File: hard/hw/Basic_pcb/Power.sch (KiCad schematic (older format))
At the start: 57 parts, among them P3 CONN_02X02, P4 CONN_02X02, U2 TPS63070

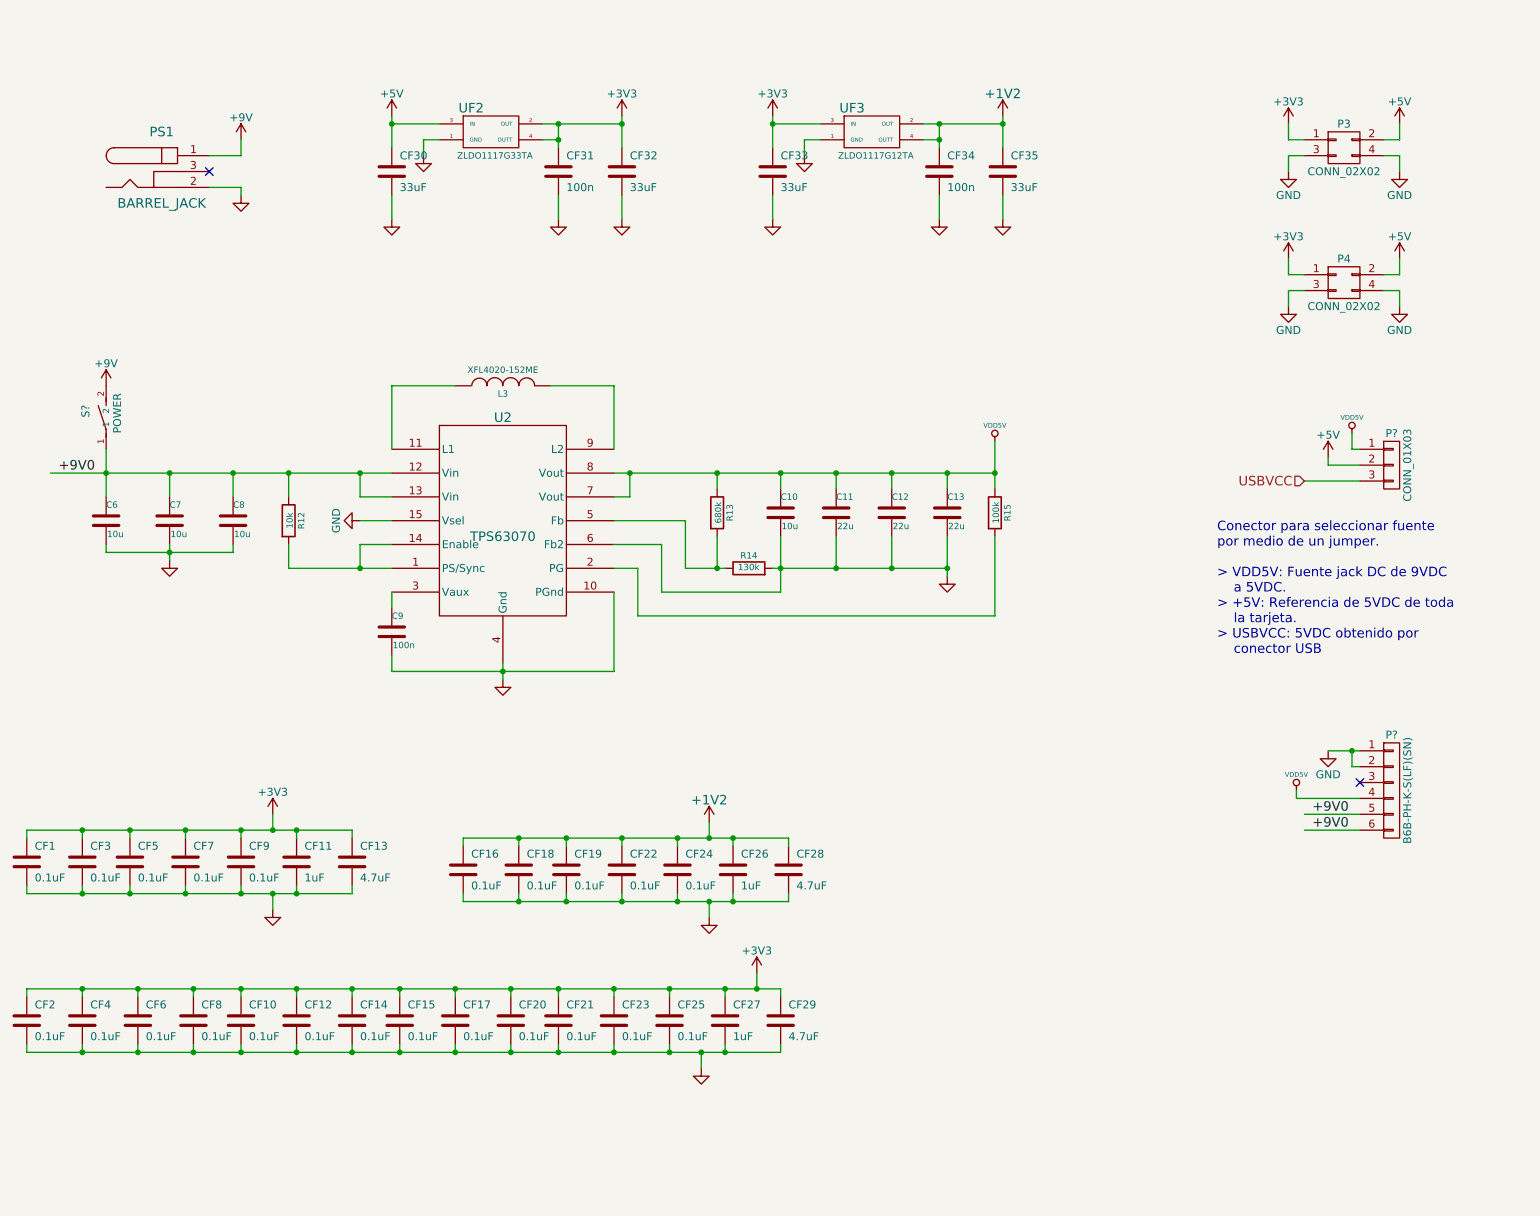
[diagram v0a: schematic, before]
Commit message: Todos los componentes en la tarjeta
by Ruben
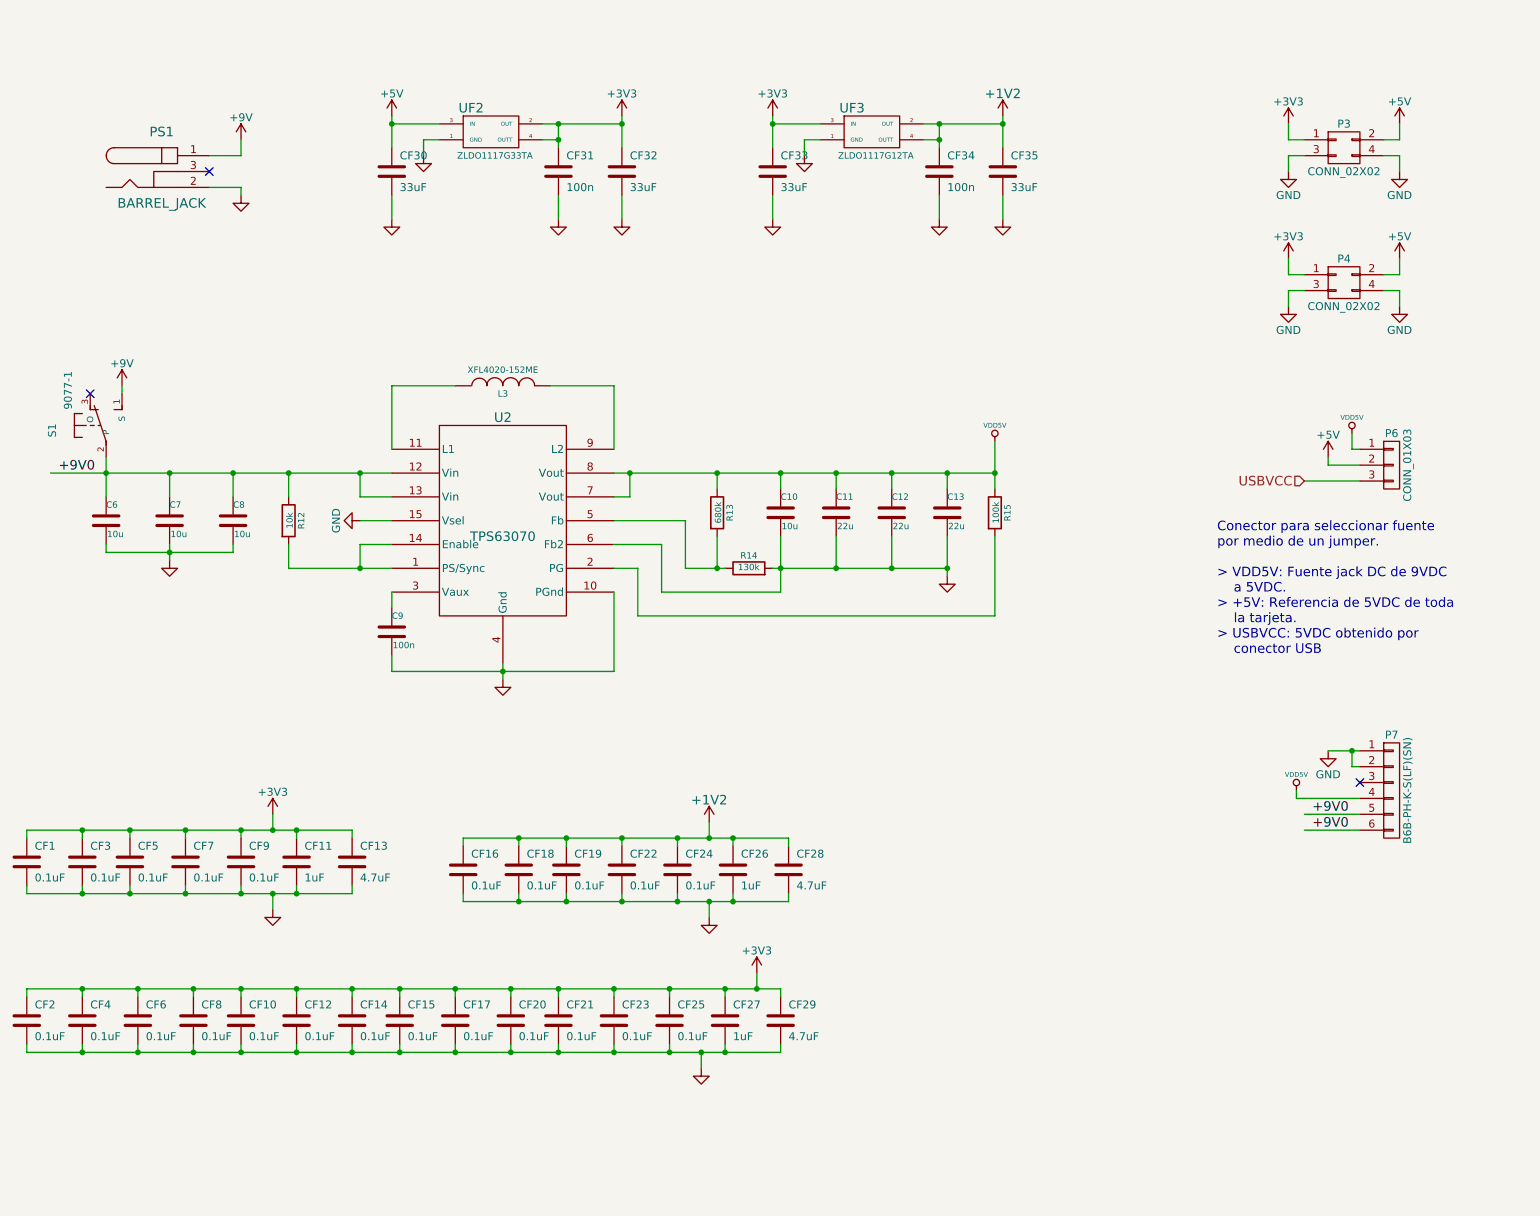
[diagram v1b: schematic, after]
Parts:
- removed S?: POWER, m-pad-2.1-SWITCH_01, symbol SWITCH_01
- added S1: 9077-1, resonator:CKCOMP-OS102011MA1QN1, symbol 9077-1
- L3: REF MOUSER (none) -> 994-XFL4020-152MEB
- P6: renamed from P?; footprint (none) -> Socket_Strips:Socket_Strip_Straight_1x03_Pitch2.54mm
- gave numbers to parts that had none: 1
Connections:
- net +9V: now also S1.1 (S)
- net +9V0: now also S1.2 (P)
- no-connect marks 2 -> 3
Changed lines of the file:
@@
 F 1 "XFL4020-152ME" V 4550 2900 40  0000 C CNN
 F 2 "resonator:XFL4020" H 4450 2900 60  0001 C CNN
-F 3 "~" H 4450 2900 60  0000 C CNN
+F 3 "http://co.mouser.com/ProductDetail/Coilcraft/XFL4020-152MEB/?qs=VJjuEbE9QBMgot7QvvqAGA%3D%3D" H 4450 2900 60  0001 C CNN
+F 4 "994-XFL4020-152MEB" V 4450 2900 60  0001 C CNN "REF MOUSER"
 	1    4450 2900
 	0    -1   -1   0
@@
 Connection ~ 7550 3450
 Wire Wire Line
-	7250 3550 7250 3450
+	7250 3450 7250 3550
 Connection ~ 7250 3450
 Wire Wire Line
-	6900 3550 6900 3450
+	6900 3450 6900 3550
 Connection ~ 6900 3450
 Wire Wire Line
-	6550 3550 6550 3450
+	6550 3450 6550 3550
 Connection ~ 6550 3450
 Wire Wire Line
-	6200 3550 6200 3450
+	6200 3450 6200 3550
 Connection ~ 6200 3450
 Wire Wire Line
-	5800 3550 5800 3450
+	5800 3450 5800 3550
 Connection ~ 5800 3450
 Wire Wire Line
@@
 	5300 4350 5300 4050
 Wire Wire Line
-	3100 3600 3100 3450
+	3100 3450 3100 3600
 Connection ~ 3100 3450
 Wire Wire Line
@@
 	1600 3450 3750 3450
 Connection ~ 1950 3450
-Wire Wire Line
-	1950 3300 1950 3600
 Wire Wire Line
 	2350 3600 2350 3450
@@
 $EndComp
 Wire Wire Line
-	5200 1400 5200 1200
+	5200 1200 5200 1400
 Wire Wire Line
 	6150 1200 6150 1400
@@
 $EndComp
 Wire Wire Line
-	7600 1400 7600 1200
+	7600 1200 7600 1400
 $Comp
 L +9V #PWR074
@@
 L +9V #PWR075
 U 1 1 58A02321
-P 1950 2900
-F 0 "#PWR075" H 1950 2750 50  0001 C CNN
-F 1 "+9V" H 1950 3040 50  0000 C CNN
-F 2 "" H 1950 2900 50  0000 C CNN
-F 3 "" H 1950 2900 50  0000 C CNN
-	1    1950 2900
+P 2050 2900
+F 0 "#PWR075" H 2050 2750 50  0001 C CNN
+F 1 "+9V" H 2050 3040 50  0000 C CNN
+F 2 "" H 2050 2900 50  0000 C CNN
+F 3 "" H 2050 2900 50  0000 C CNN
+	1    2050 2900
 	1    0    0    -1
 $EndComp
@@
 	6050 6700 6050 6600
 $Comp
-L CONN_01X06 P?
+L CONN_01X06 P7
 U 1 1 58B0BB4F
 P 10050 5450
-F 0 "P?" H 10050 5800 50  0000 C CNN
+F 0 "P7" H 10050 5800 50  0000 C CNN
 F 1 "B6B-PH-K-S(LF)(SN)" V 10150 5450 50  0000 C CNN
 F 2 "Connectors_JST:JST_PH_B6B-PH-K_06x2.00mm_Straight" H 10050 5450 50  0001 C CNN
@@
 $EndComp
 $Comp
-L CONN_01X03 P?
+L CONN_01X03 P6
 U 1 1 58B0D54B
 P 10050 3400
-F 0 "P?" H 10050 3600 50  0000 C CNN
+F 0 "P6" H 10050 3600 50  0000 C CNN
 F 1 "CONN_01X03" V 10150 3400 50  0000 C CNN
-F 2 "" H 10050 3400 50  0000 C CNN
+F 2 "Socket_Strips:Socket_Strip_Straight_1x03_Pitch2.54mm" H 10050 3400 50  0001 C CNN
 F 3 "" H 10050 3400 50  0000 C CNN
 	1    10050 3400
@@
 $EndComp
 $Comp
-L GND #PWR?
+L GND #PWR093
 U 1 1 58B125AC
 P 9650 5200
-F 0 "#PWR?" H 9650 4950 50  0001 C CNN
+F 0 "#PWR093" H 9650 4950 50  0001 C CNN
 F 1 "GND" H 9650 5050 50  0000 C CNN
 F 2 "" H 9650 5200 50  0000 C CNN
@@
 +9V0
 $Comp
-L VDD5V #PWR?
+L VDD5V #PWR094
 U 1 1 58B1B9B1
 P 9450 5450
-F 0 "#PWR?" H 9450 5550 30  0001 C CNN
+F 0 "#PWR094" H 9450 5550 30  0001 C CNN
 F 1 "VDD5V" H 9450 5550 30  0000 C CNN
 F 2 "" H 9450 5450 60  0000 C CNN
@@
 	9450 5500 9450 5450
 Wire Wire Line
-	9850 5200 9650 5200
+	9650 5200 9850 5200
 Wire Wire Line
 	9850 5300 9800 5300
@@
 	9800 5300 9800 5200
 Connection ~ 9800 5200
-$Comp
-L SWITCH_01 S?
-U 1 1 58B0E065
-P 1950 3100
-F 0 "S?" V 1850 3100 50  0000 L BNN
-F 1 "POWER" V 2050 3000 50  0000 L BNN
-F 2 "m-pad-2.1-SWITCH_01" H 1950 3250 50  0001 C CNN
-F 3 "" H 1950 3100 60  0001 C CNN
-	1    1950 3100
-	1    0    0    -1
-$EndComp
+Wire Wire Line
+	1950 3350 1950 3600
+$Comp
+L 9077-1 S1
+U 1 1 58B4DBD3
+P 1950 3150
+F 0 "S1" V 1640 3075 50  0000 L BNN
+F 1 "9077-1" V 1740 3250 50  0000 L BNN
+F 2 "resonator:CKCOMP-OS102011MA1QN1" H 1950 3300 50  0001 C CNN
+F 3 "http://www.ckswitches.com/media/1428/os.pdf" H 1950 3150 60  0001 C CNN
+F 4 "CKN9559-ND" V 1950 3150 60  0001 C CNN "REF DIGIKEY"
+	1    1950 3150
+	1    0    0    -1
+$EndComp
+Wire Wire Line
+	2050 2900 2050 2950
+NoConn ~ 1850 2950
 $EndSCHEMATC

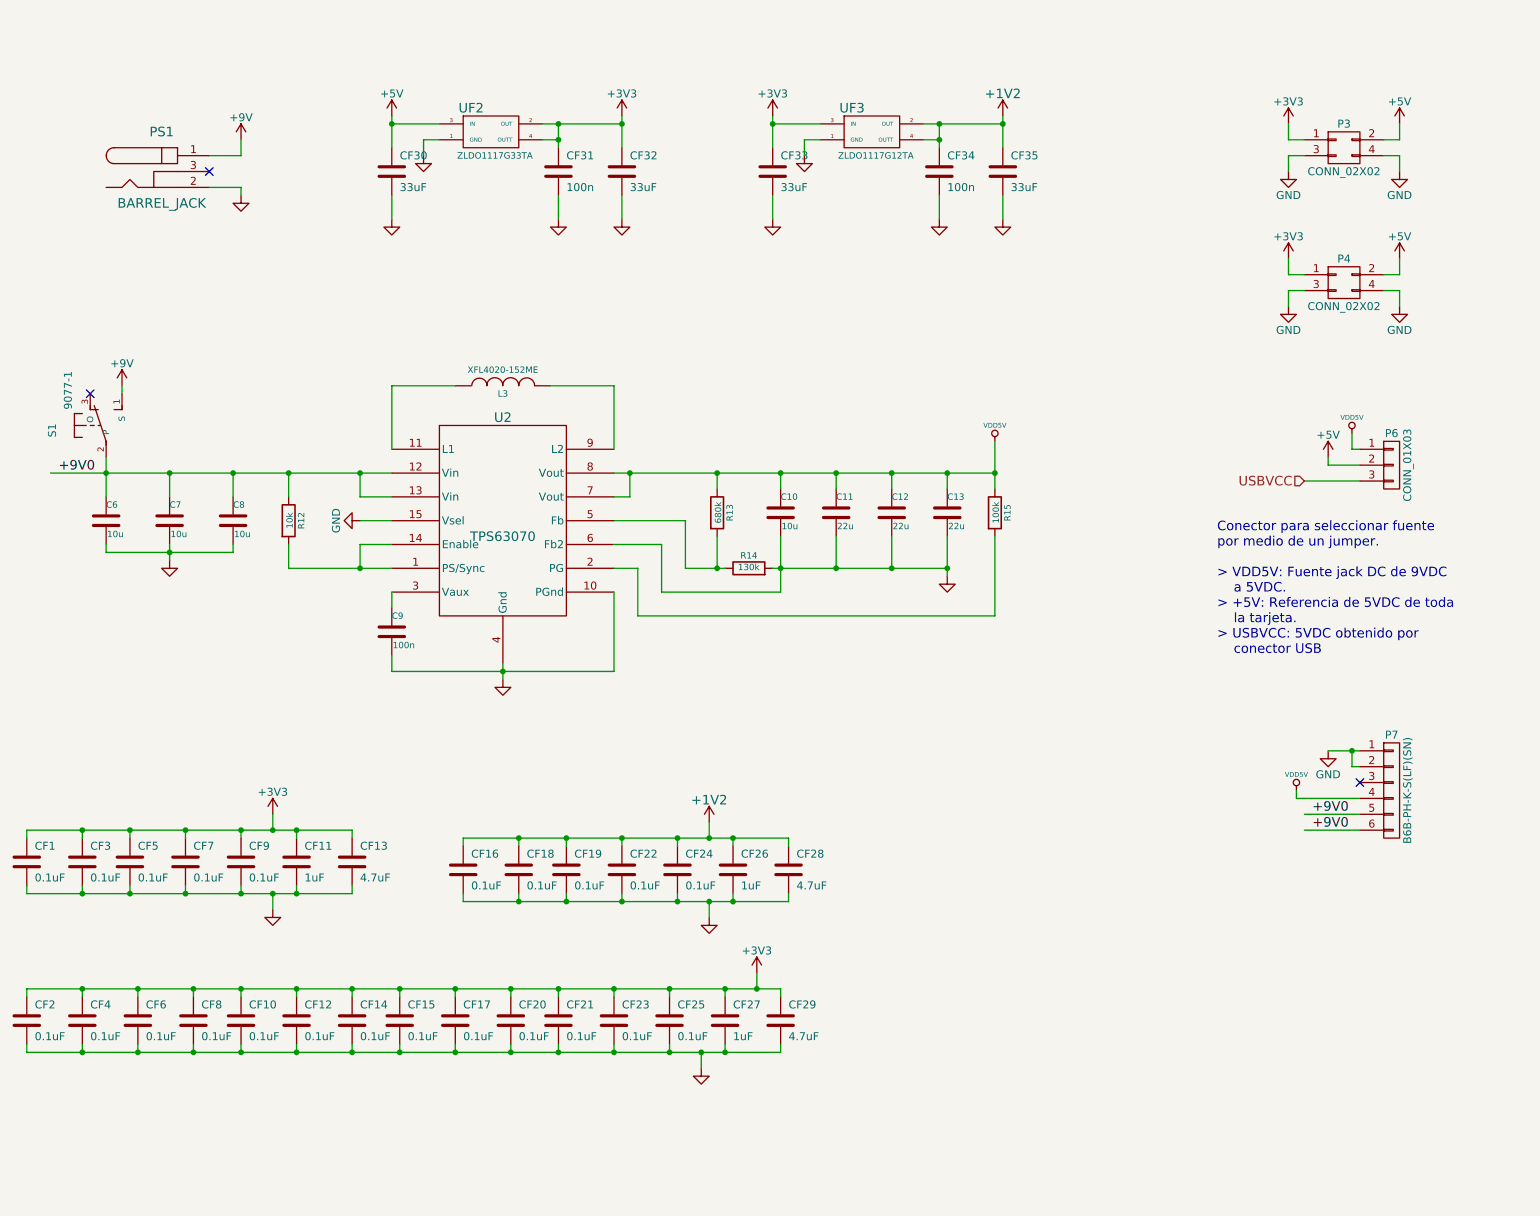
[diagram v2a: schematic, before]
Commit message: Actualización K3
by Ruben
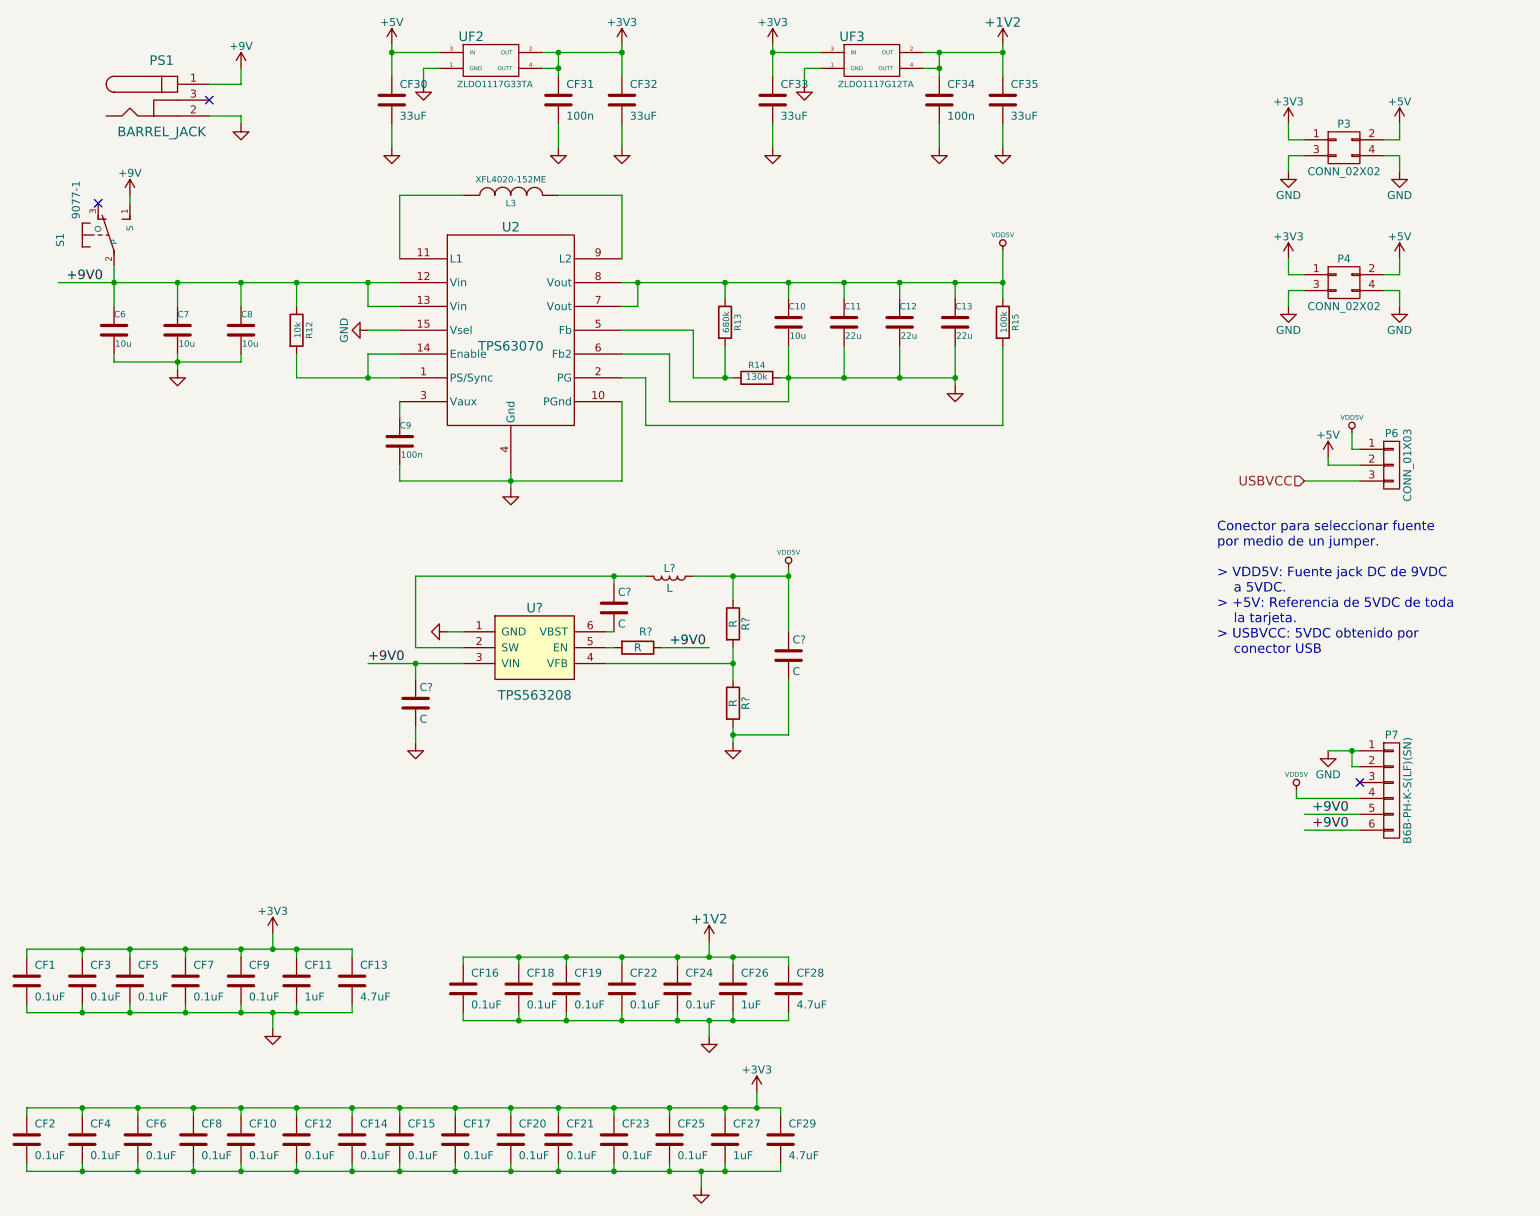
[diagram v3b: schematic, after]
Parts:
- added C? (x3): C, symbol C
- added L?: L, symbol L
- added R? (x3): R, symbol R
- added U?: TPS563208, TO_SOT_Packages_SMD:SOT-23-6, symbol TPS563208
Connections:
- net +9V0: now also C?.1, R?.1, U?.3 (VIN)
- net GND: now also C?.2, C?.2, R?.2, U?.1 (GND)
- net VDD5V: now also C?.1, L?.1, R?.1
- new net: C?.1, L?.2, U?.2 (SW)
- new net: R?.1, R?.2, U?.4 (VFB)
- new net: R?.2, U?.5 (EN)
- new net: C?.2, U?.6 (VBST)
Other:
- moved on the sheet: C10, C11, C12, C13, C6, C7, C8, C9, CF1, CF10, CF11, CF12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
